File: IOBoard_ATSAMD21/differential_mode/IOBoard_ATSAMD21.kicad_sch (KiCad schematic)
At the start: 40 parts, among them J1 Conn_PIC_ICSP_ICD, J13 Eurorack_Mono_Jack, J2 Conn_01x04_Male, SW1 EG_1218, SW2 EG_1218, SW3 EG_1218, SW4 EG_1218, U1 ATSAMD21G18A-A, U2 AP2112K-3.3

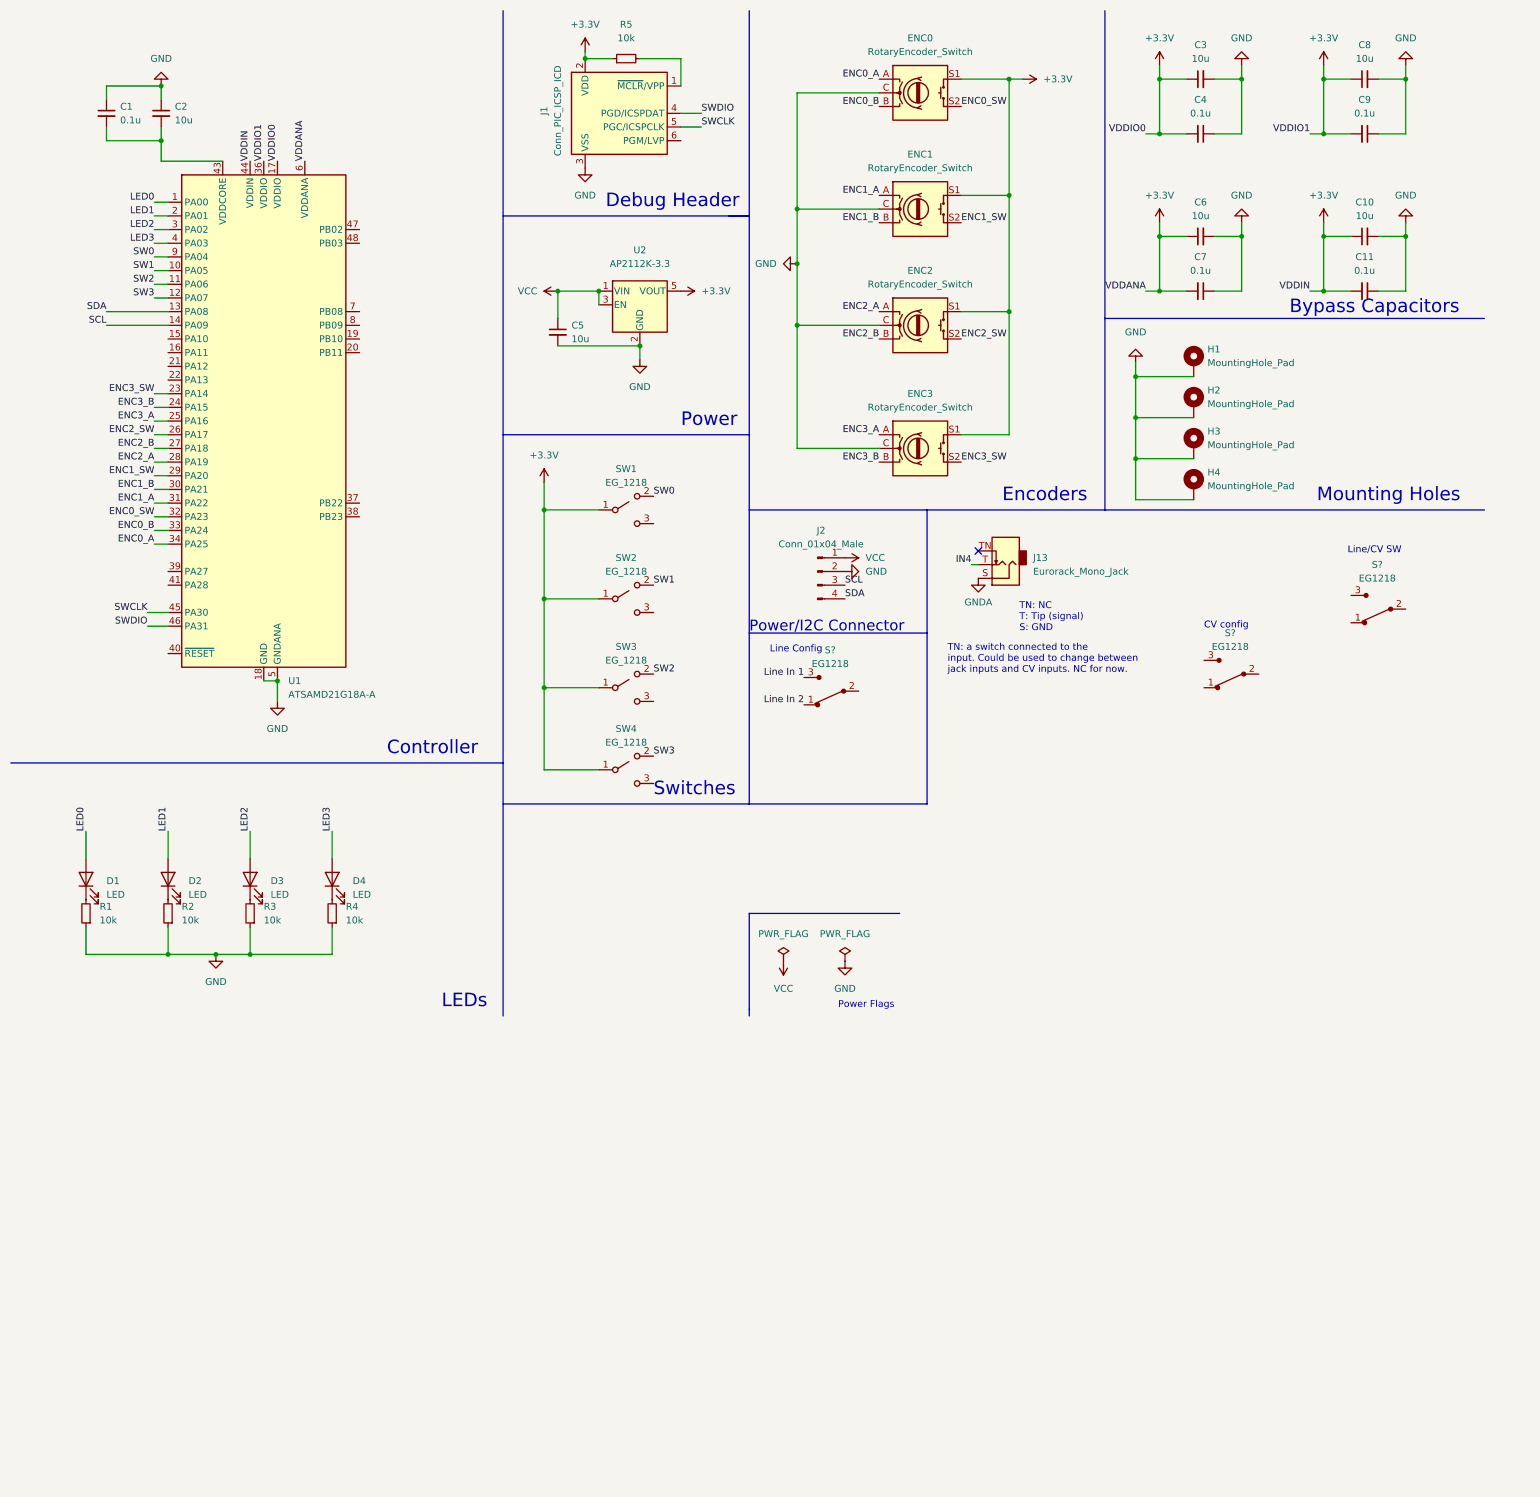
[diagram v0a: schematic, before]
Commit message: giving up on differential for now
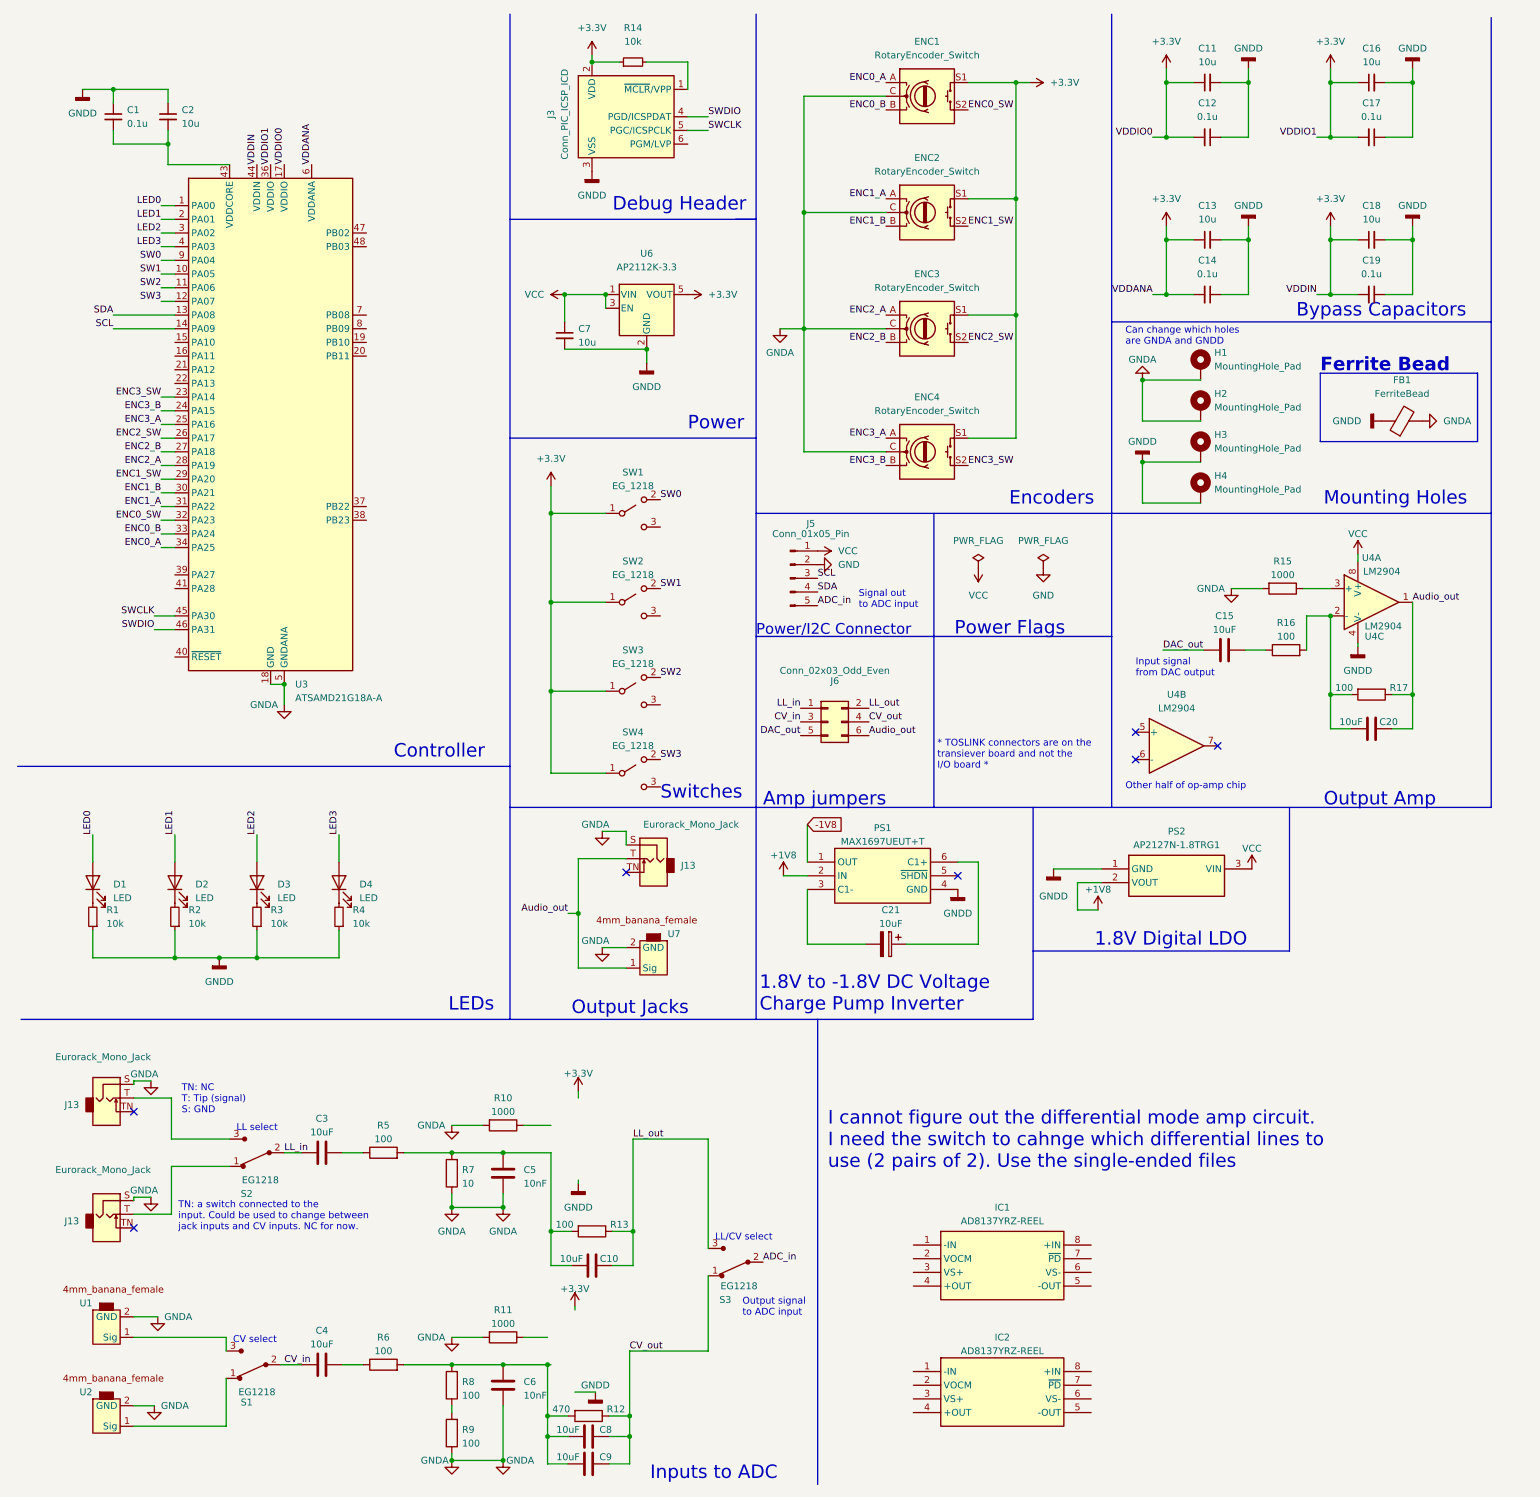
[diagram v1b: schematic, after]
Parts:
- removed C10, C3, C5, C6, C8: 10u, Capacitor_SMD:C_0603_1608Metric, symbol Device:C_Small
- removed C4, C9: 0.1u, Capacitor_SMD:C_0603_1608Metric, symbol Device:C_Small
- removed ENC0: RotaryEncoder_Switch, custom_lib:PEC12R-3217F-S0024-ND, symbol Device:RotaryEncoder_Switch
- removed J1: Conn_PIC_ICSP_ICD, Connector_PinHeader_2.54mm:PinHeader_1x06_P2.54mm_Vertical, symbol Connector:Conn_PIC_ICSP_ICD
- removed J13: Eurorack_Mono_Jack, winterbloom:AudioJack_WQP518MA, symbol winterbloom:Eurorack_Mono_Jack
- removed J2: Conn_01x04_Male, Connector_PinHeader_2.54mm:PinHeader_1x04_P2.54mm_Vertical, symbol Connector:Conn_01x04_Male
- removed R5: 10k, Resistor_SMD:R_0603_1608Metric, symbol Device:R_Small
- removed S? (x3): EG1218, digikey-footprints:Switch_Slide_11.6x4mm_EG1218, symbol dk_Slide-Switches:EG1218
- removed U1: ATSAMD21G18A-A, Package_QFP:TQFP-48_7x7mm_P0.5mm, symbol MCU_Microchip_SAMD:ATSAMD21G18A-A
- removed U2: AP2112K-3.3, Package_TO_SOT_SMD:SOT-23-5, symbol Regulator_Linear:AP2112K-3.3
- added C10, C15, C20, C3, C4, C8, C9: 10uF, Capacitor_SMD:C_0603_1608Metric, symbol Device:C
- added C12, C14, C17, C19: 0.1u, Capacitor_SMD:C_0603_1608Metric, symbol Device:C_Small
- added C13, C16, C18: 10u, Capacitor_SMD:C_0603_1608Metric, symbol Device:C_Small
- added C21: 10uF, symbol Device:C_Polarized
- added C5, C6: 10nF, Capacitor_SMD:C_0603_1608Metric, symbol Device:C
- added ENC4: RotaryEncoder_Switch, custom_lib:PEC12R-3217F-S0024-ND, symbol Device:RotaryEncoder_Switch
- added FB1: FerriteBead, Inductor_SMD:L_0603_1608Metric_Pad1.05x0.95mm_HandSolder, symbol Device:FerriteBead
- added IC1, IC2: AD8137YRZ-REEL, SOIC127P600X175-8N, symbol AD8137YRZ-REEL:AD8137YRZ-REEL
- added J13 (x3): Eurorack_Mono_Jack, winterbloom:AudioJack_WQP518MA, symbol winterbloom:Eurorack_Mono_Jack
- added J3: Conn_PIC_ICSP_ICD, Connector_PinHeader_2.54mm:PinHeader_1x06_P2.54mm_Vertical, symbol Connector:Conn_PIC_ICSP_ICD
- added J5: Conn_01x05_Pin, symbol Connector:Conn_01x05_Pin
- added J6: Conn_02x03_Odd_Even, symbol Connector_Generic:Conn_02x03_Odd_Even
- added PS1: MAX1697UEUT+T, SOT95P280X145-6N, symbol custom_lib:MAX1697UEUT+T
- added PS2: AP2127N-1.8TRG1, SOT95P240X120-3N, symbol AP2127N-1_8TRG1:AP2127N-1.8TRG1
- added R10, R11, R15: 1000, Resistor_SMD:R_0603_1608Metric, symbol Device:R
- added R12: 470, Resistor_SMD:R_0603_1608Metric, symbol Device:R
- added R13, R16, R17, R5, R6, R8, R9: 100, Resistor_SMD:R_0603_1608Metric, symbol Device:R
- added R14: 10k, Resistor_SMD:R_0603_1608Metric, symbol Device:R_Small
- added R7: 10, Resistor_SMD:R_0603_1608Metric, symbol Device:R
- added S1, S2, S3: EG1218, digikey-footprints:Switch_Slide_11.6x4mm_EG1218, symbol dk_Slide-Switches:EG1218
- added U1, U2, U7: ~, custom_lib:4mm_banana_female, symbol custom_lib:4mm_female_banana
- added U3: ATSAMD21G18A-A, Package_QFP:TQFP-48_7x7mm_P0.5mm, symbol MCU_Microchip_SAMD:ATSAMD21G18A-A
- added U4: LM2904, symbol Amplifier_Operational:LM2904
- added U6: AP2112K-3.3, Package_TO_SOT_SMD:SOT-23-5, symbol Regulator_Linear:AP2112K-3.3
- C11, C7: value 0.1u -> 10u
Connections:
- net +3.3V: now also C11.1, C12.2, C13.1, C14.2, C16.1, C17.2, C18.1, C19.2, ENC4.S1, J3.2 (VDD), R14.1, U3.17 (VDDIO), U3.36 (VDDIO), U3.44 (VDDIN), U3.6 (VDDANA), U6.5 (VOUT); no longer C11.2, C7.2
- net ENC0_A: now also ENC1.A, U3.34 (PA25)
- net ENC0_B: now also ENC1.B, U3.33 (PA24)
- net ENC0_SW: now also ENC1.S2, U3.32 (PA23)
- net ENC1_A: now also ENC2.A, U3.31 (PA22); no longer ENC1.A
- net ENC1_B: now also ENC2.B, U3.30 (PA21); no longer ENC1.B
- net ENC1_SW: now also ENC2.S2, U3.29 (PA20); no longer ENC1.S2
- net ENC2_A: now also ENC3.A, U3.28 (PA19); no longer ENC2.A
- net ENC2_B: now also ENC3.B, U3.27 (PA18); no longer ENC2.B
- net ENC2_SW: now also ENC3.S2, U3.26 (PA17); no longer ENC2.S2
- net ENC3_A: now also ENC4.A, U3.25 (PA16); no longer ENC3.A
- net ENC3_B: now also ENC4.B, U3.24 (PA15); no longer ENC3.B
- net ENC3_SW: now also ENC4.S2, U3.23 (PA14); no longer ENC3.S2
- net GND: now also J5.2 (Pin_2); no longer C1.1, C11.1, C2.1, C7.1, ENC1.C, ENC2.C, ENC3.C, H1.1, H2.1, H3.1, H4.1, R1.1, R2.1, R3.1, R4.1
- net GNDA: now also ENC1.C, ENC2.C, ENC3.C, H1.1, H2.1, C5.1, C6.1, ENC4.C, FB1.2, J13.S (Sleeve), J13.S (Sleeve), J13.S (Sleeve), R10.2, R11.2, R15.2, R7.1, R9.1, U1.2 (GND), U2.2 (GND), U3.18 (GND), U3.35 (GND), U3.42 (GND), U3.5 (GNDANA), U7.2 (GND)
- net LED0: now also U3.1 (PA00)
- net LED1: now also U3.2 (PA01)
- net LED2: now also U3.3 (PA02)
- net LED3: now also U3.4 (PA03)
- net SCL: now also J5.3 (Pin_3), U3.14 (PA09)
- net SDA: now also J5.4 (Pin_4), U3.13 (PA08)
- net SW0: now also U3.9 (PA04)
- net SW1: now also U3.10 (PA05)
- net SW2: now also U3.11 (PA06)
- net SW3: now also U3.12 (PA07)
- net SWCLK: now also J3.5 (PGC/ICSPCLK), U3.45 (PA30)
- net SWDIO: now also J3.4 (PGD/ICSPDAT), U3.46 (PA31)
- net VCC: now also C7.1, J5.1 (Pin_1), PS2.3 (VIN), U4.8 (V+), U6.1 (VIN), U6.3 (EN)
- net at C1.2, C2.2: now also U3.43 (VDDCORE)
- new net: C4.2, R6.1
- new net: C6.2, C8.2, C9.2, R12.2, R6.2, R8.2
- new net: R8.1, R9.2
- new net: J13.T (Tip), S2.1
- new net: C10.2, C5.2, R13.2, R5.2, R7.2
- new net: S1.1, U2.1 (Sig)
- new net: C3.2, R5.1
- new net: J3.1 (~{MCLR}/VPP), R14.2
- new net: C20.2, R16.2, R17.2, U4.2 (-)
- new net: R15.1, U4.3 (+)
- new net: C21.2, PS1.3 (C1-)
- new net: C21.1, PS1.6 (C1+)
- new net: S1.3, U1.1 (Sig)
- new net: J13.T (Tip), S2.3
- new net: C15.2, R16.1
- new net +1V8: PS1.2 (IN), PS2.2 (VOUT)
- new net -1V8: PS1.1 (OUT)
- new net ADC_in: J5.5 (Pin_5), S3.2
- new net Audio_out: C20.1, J13.T (Tip), J6.6 (Pin_6), R17.1, U4.1, U7.1 (Sig)
- new net CV_in: C4.1, J6.3 (Pin_3), S1.2
- new net CV_out: C8.1, C9.1, J6.4 (Pin_4), R12.1, S3.1
- new net DAC_out: C15.1, J6.5 (Pin_5)
- new net GNDD: C1.1, C11.2, C12.1, C13.2, C14.1, C16.2, C17.1, C18.2, C19.1, C2.1, C7.2, FB1.1, H3.1, H4.1, J3.3 (VSS), PS1.4 (GND), PS2.1 (GND), R1.1, R2.1, R3.1, R4.1, U4.4 (V-), U6.2 (GND)
- new net LL_in: C3.1, J6.1 (Pin_1), S2.2
- new net LL_out: C10.1, J6.2 (Pin_2), R13.1, S3.3
- no-connect marks 1 -> 7
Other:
- note added: "* TOSLINK connectors are on the transiever board and not the I/O board *"
- note added: "1.8V Digital LDO"
- note added: "1.8V to -1.8V DC Voltage Charge Pump Inverter"
- note added: "Amp jumpers"
- note added: "CV select"
- note added: "Can change which holes are GNDA and GNDD"
- note added: "Ferrite Bead"
- note added: "I cannot figure out the differential mode amp circuit. I need the switch to cahnge which differential lines to use (2 pairs of 2). Use the single-ended files"
- note added: "Input signal from DAC output"
- note added: "Inputs to ADC"
- note added: "LL select"
- note added: "LL/CV select"
- note added: "Other half of op-amp chip"
- note added: "Output Amp"
- note added: "Output Jacks"
- note added: "Output signal to ADC input"
- note added: "Signal out to ADC input"
- note removed: "CV config"
- note removed: "Line Config"
- note removed: "Line/CV SW"
